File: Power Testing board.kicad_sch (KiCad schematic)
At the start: 13 parts, among them J1 Conn_01x26_Pin, J2 Conn_01x26_Pin, J3 Conn_01x26_Pin, J4 Conn_01x26_Pin, U1 INA260, U2 INA260, U3 INA260, U4 INA260, U5 TPS26631RGE, U6 TPS26631RGE, U7 TPS26631RGE, U8 TPS26631RGE

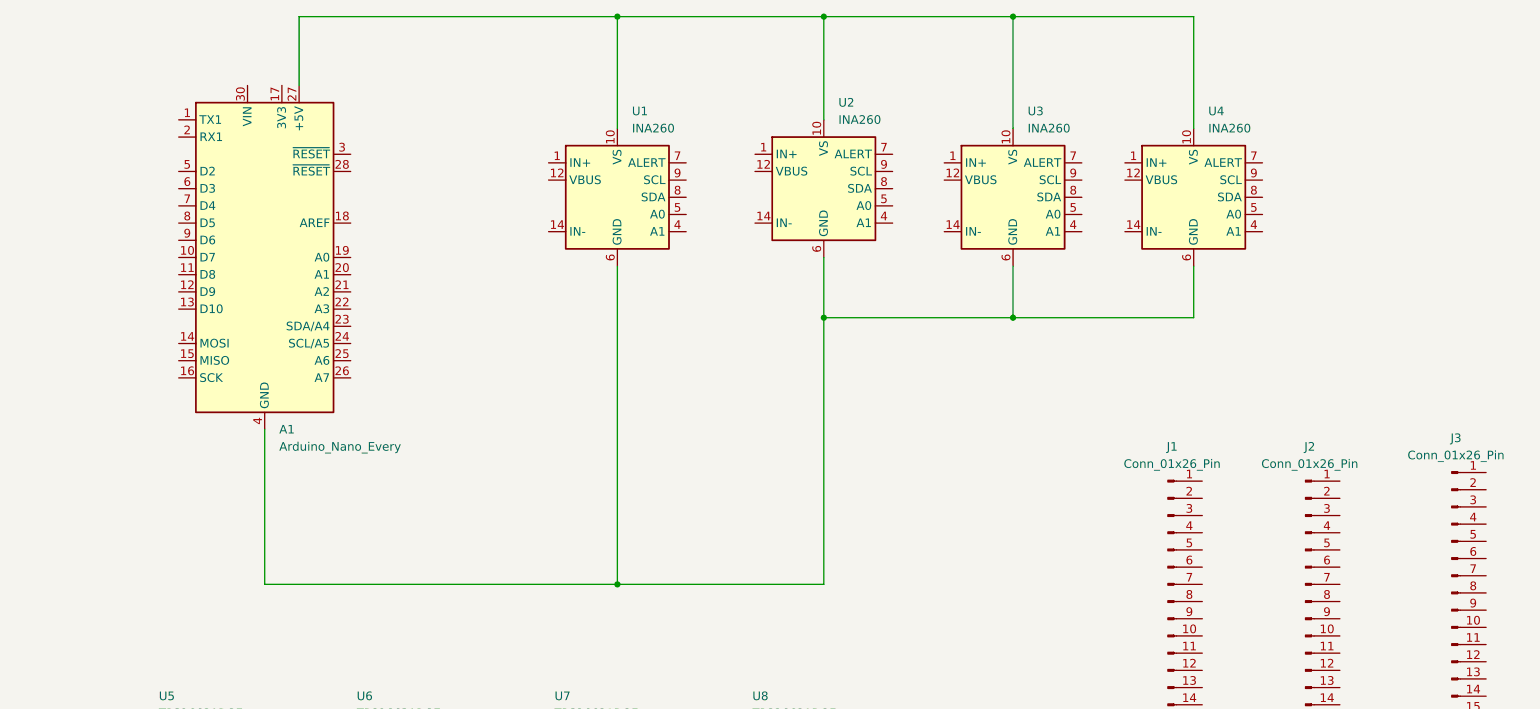
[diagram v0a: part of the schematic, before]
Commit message: GN
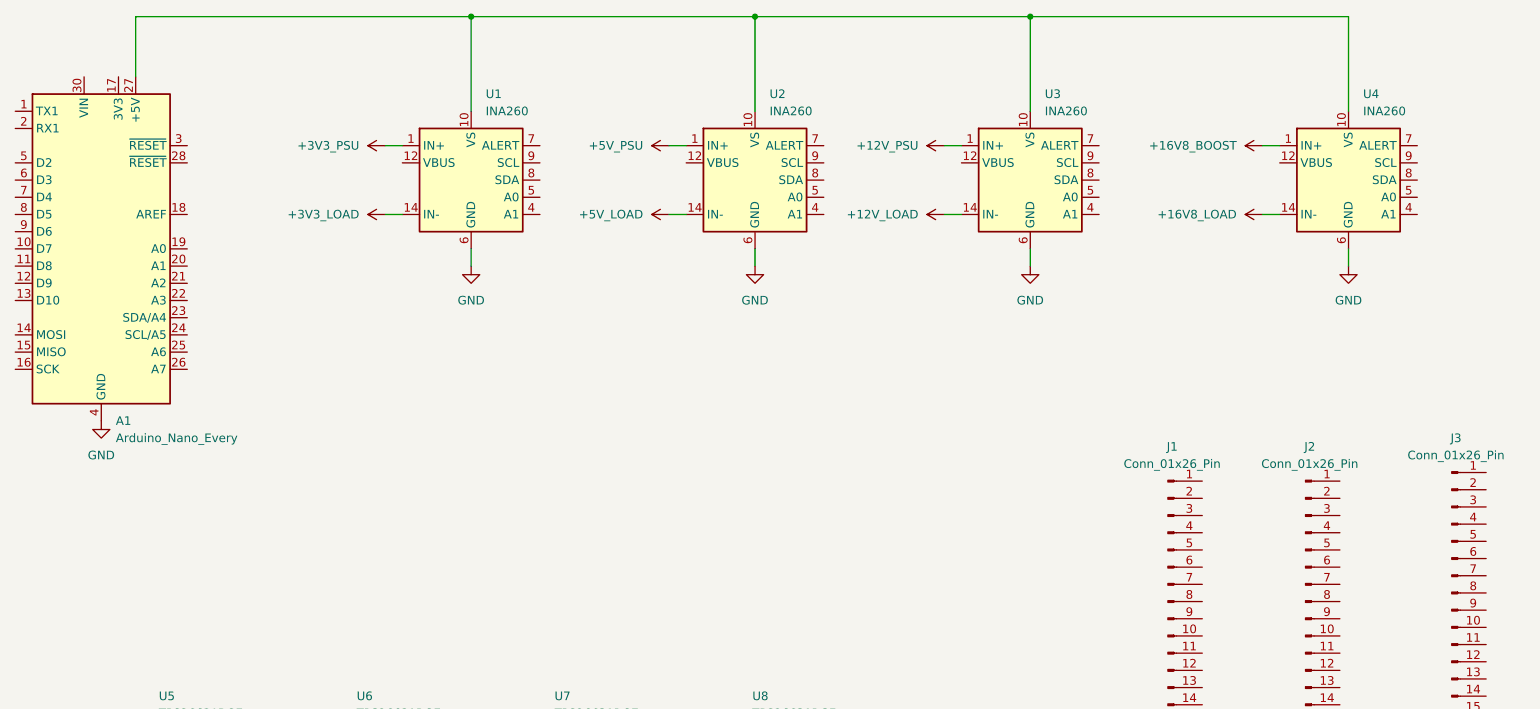
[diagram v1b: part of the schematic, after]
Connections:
- net GND: now also A1.29 (GND), A1.4 (GND), U1.11 (GND), U1.6 (GND), U2.11 (GND), U2.6 (GND), U3.11 (GND), U3.6 (GND), U4.11 (GND), U4.6 (GND)
- net +3V3_PSU: now reaches U1.1 (IN+), U1.2 (IN+), U1.3 (IN+)
- net +3V3_LOAD: now reaches U1.14 (IN-), U1.15 (IN-), U1.16 (IN-)
- net +5V_PSU: now reaches U2.1 (IN+), U2.2 (IN+), U2.3 (IN+)
- net +5V_LOAD: now reaches U2.14 (IN-), U2.15 (IN-), U2.16 (IN-)
- net +16V8_BOOST: now reaches U4.1 (IN+), U4.2 (IN+), U4.3 (IN+)
- net +16V8_LOAD: now reaches U4.14 (IN-), U4.15 (IN-), U4.16 (IN-)
- net +12V_PSU: now reaches U3.1 (IN+), U3.2 (IN+), U3.3 (IN+)
- net +12V_LOAD: now reaches U3.14 (IN-), U3.15 (IN-), U3.16 (IN-)
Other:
- moved on the sheet: A1, U1, U2, U3, U4

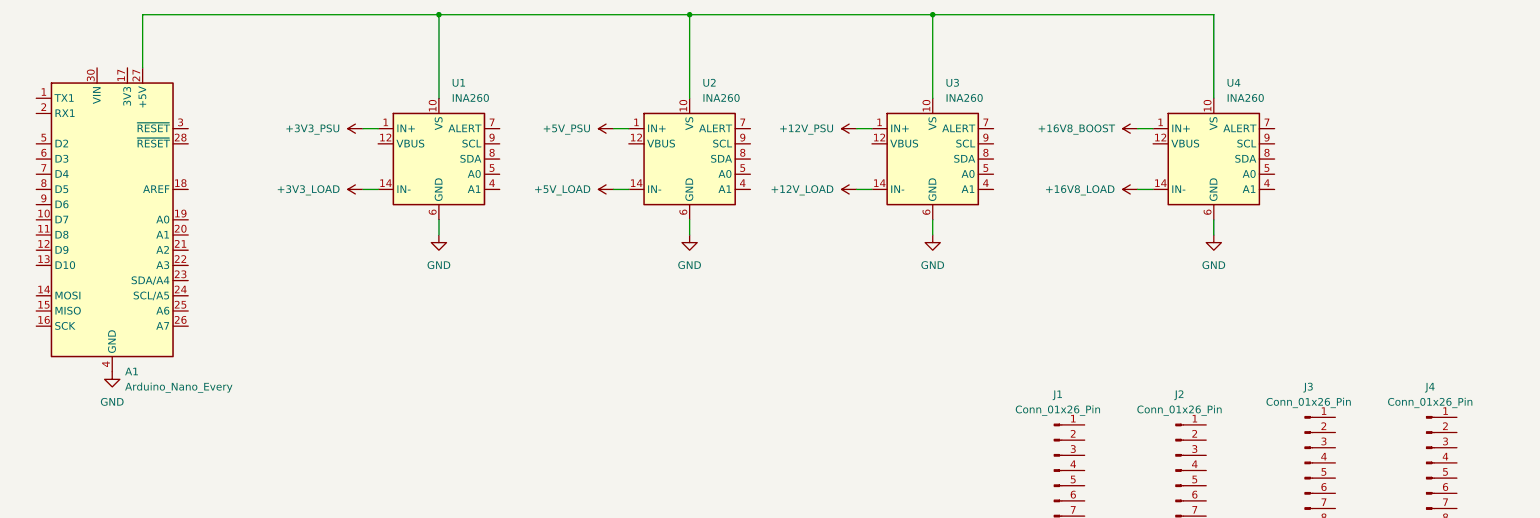
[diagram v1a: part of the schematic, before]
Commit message: i2C
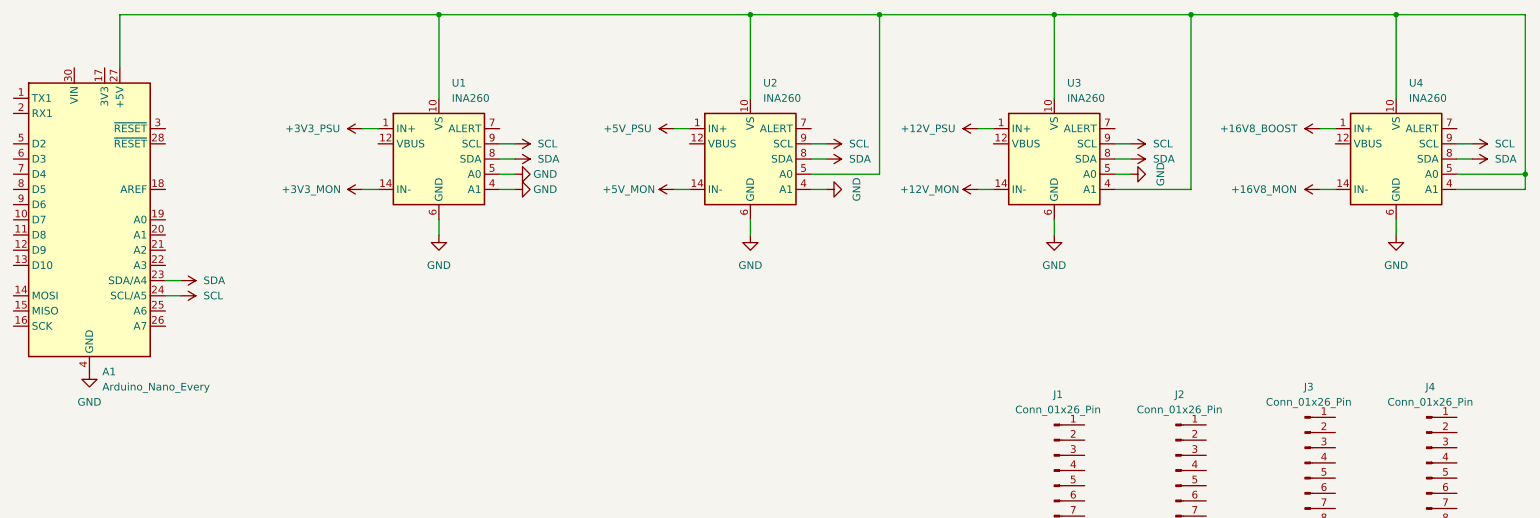
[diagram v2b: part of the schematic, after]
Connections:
- net GND: now also U1.4 (A1), U1.5 (A0), U2.4 (A1), U3.5 (A0)
- net at A1.27 (+5V), U1.10 (VS), U2.10 (VS)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: now also U2.5 (A0), U3.4 (A1), U4.4 (A1), U4.5 (A0)
- net SDA: now reaches U1.8 (SDA)
- net SDA: now also A1.23 (SDA/A4), U2.8 (SDA), U3.8 (SDA), U4.8 (SDA)
- net SCL: now reaches U1.9 (SCL)
- net SCL: now also A1.24 (SCL/A5), U2.9 (SCL), U3.9 (SCL), U4.9 (SCL)
- net +12V_LOAD renamed +12V_MON
- net +16V8_LOAD renamed +16V8_MON
- net +3V3_LOAD renamed +3V3_MON
- net +5V_LOAD renamed +5V_MON
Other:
- moved on the sheet: A1, U2, U3, U4

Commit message: New pages
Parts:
- removed U5, U6, U7, U8: TPS26631RGE, Package_DFN_QFN:Texas_RGE0024H_VQFN-24-1EP_4x4mm_P0.5mm_EP2.7x2.7mm_ThermalVias, symbol Power_Management:TPS26631RGE
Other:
- added sheet Headers (Headers.kicad_sch)
- added sheet Untitled Sheet (untitled.kicad_sch)
- company: (none) -> CSULB SHARKSAT TEAM
- title: (none) -> Power Testing Board
